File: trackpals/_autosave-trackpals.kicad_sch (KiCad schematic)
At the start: 103 parts, among them J1 CONUFL001-SMD-T, J2 Conn_01x02_Socket, J3 Battery Connector, J4 CONUFL001-SMD-T, Q1 BC848, Q2 AO4459, Q3 BSS138, Q4 BSS138, SW1 SW_Push, SW2 SW_Push, SW3 SW_Push, U1 TXS0102DCT, U2 BQ24040DSQR, U3 TPS73733DCQR, U4 TPL5110, U5 CH340C, U6 SIM800C, U7 ESP32-WROOM-32, U8 NEO-6M-GPS, U9 HK24C32HA-USR-B

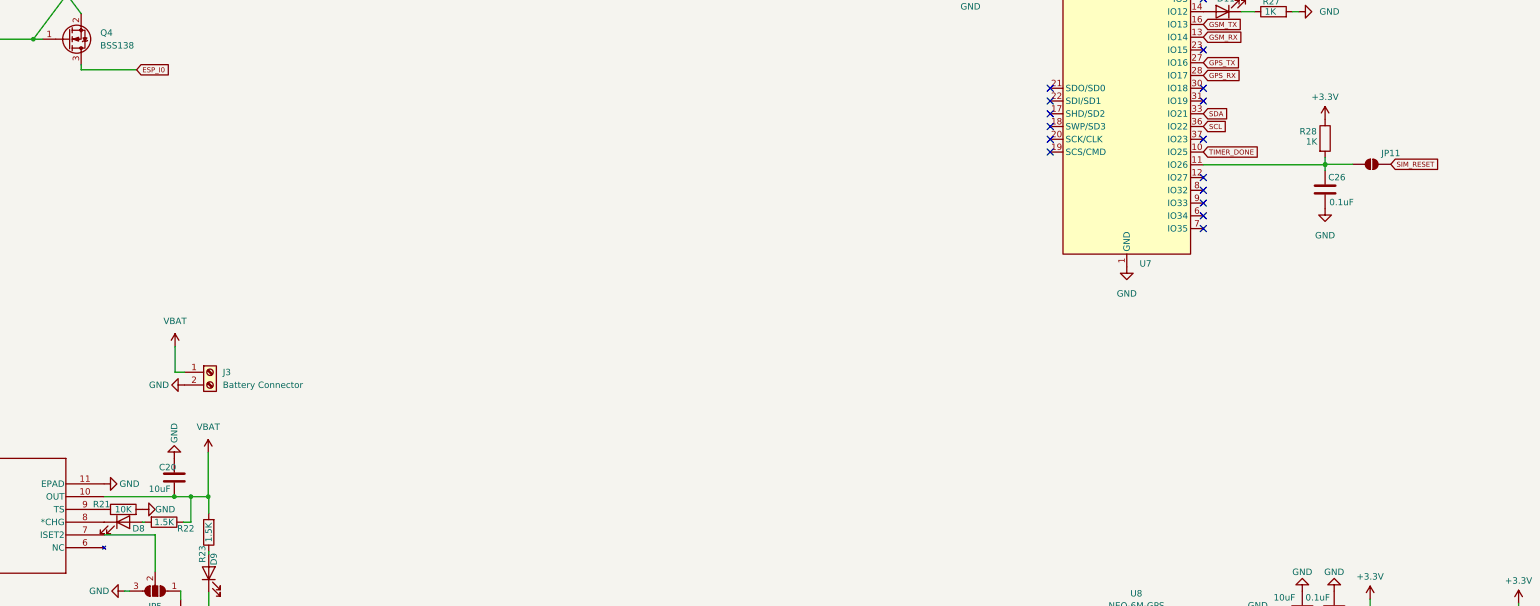
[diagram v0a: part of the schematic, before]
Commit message: -done placement ng pcb
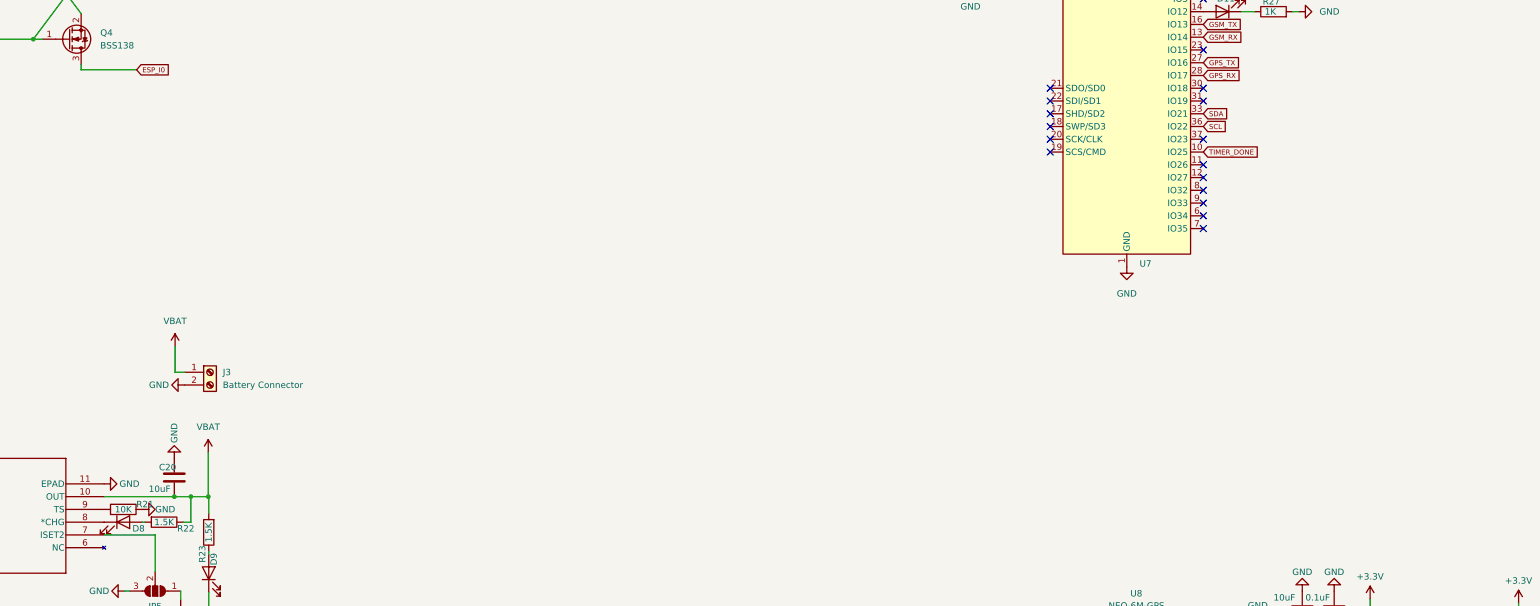
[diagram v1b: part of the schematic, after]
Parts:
- removed C26: 0.1uF, Capacitor_SMD:C_0805_2012Metric_Pad1.18x1.45mm_HandSolder, symbol Device:C
- removed JP11: SolderJumper_2_Open, Jumper:SolderJumper-2_P1.3mm_Open_Pad1.0x1.5mm, symbol Jumper:SolderJumper_2_Open
- removed R28: 1K, Resistor_SMD:R_0603_1608Metric_Pad0.98x0.95mm_HandSolder, symbol Device:R
- D12: footprint Diode_THT:D_DO-41_SOD81_P10.16mm_Horizontal -> Diode_SMD:D_SOD-123F
- J2: footprint Connector_PinHeader_2.54mm:PinHeader_1x02_P2.54mm_Vertical -> Jumper:SolderJumper-2_P1.3mm_Open_Pad1.0x1.5mm
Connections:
- net GND: now also R21.1; no longer R21.2
- net at U2.9 (TS): now also R21.2; no longer R21.1
- no-connect marks 59 -> 60
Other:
- moved on the sheet: R21
